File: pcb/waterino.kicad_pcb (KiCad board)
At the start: 2 copper layers, 49 x 84 mm, 50 parts, among them IC1 ATMEGA168A-P, P6 CONN_01X04, U1 LM7805CT, U2 MIC94090, U3 MAX6817, Y1 Crystal

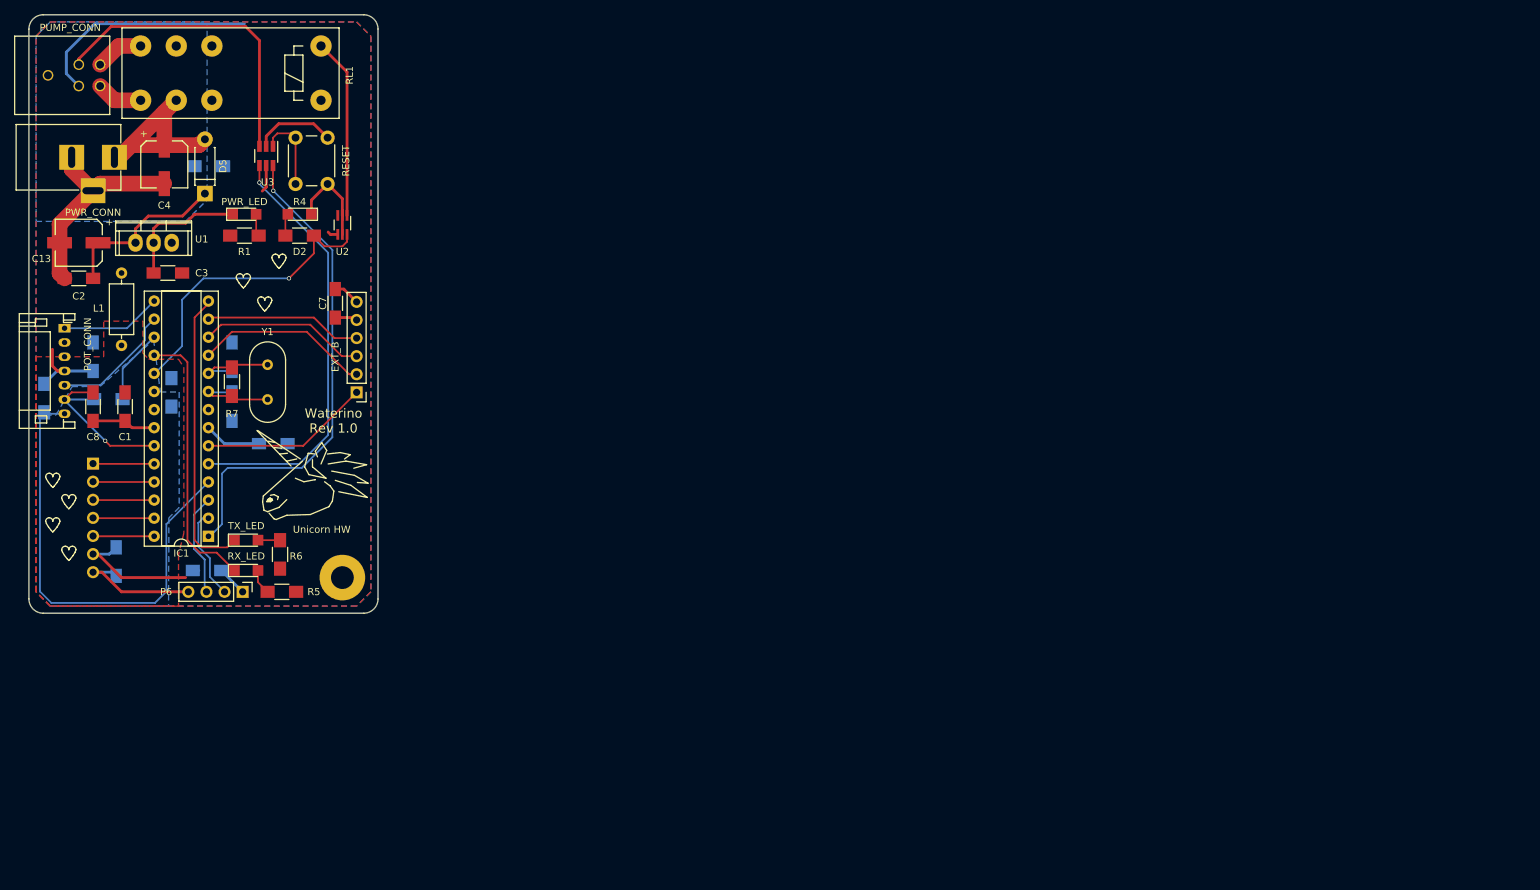
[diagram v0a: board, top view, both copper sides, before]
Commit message: wip
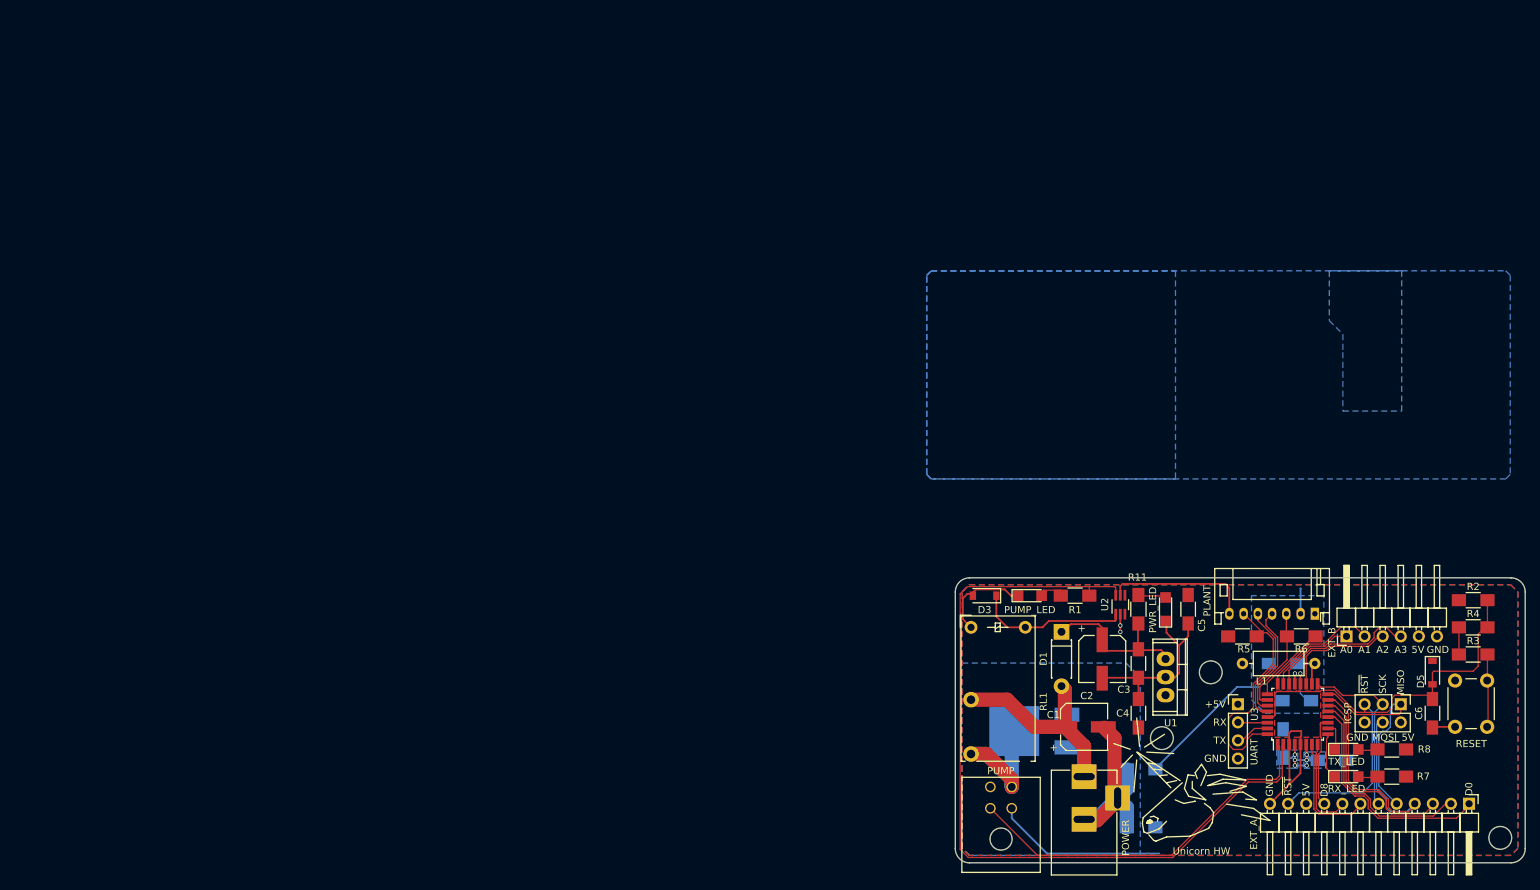
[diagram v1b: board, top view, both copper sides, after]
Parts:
- removed C10: 100nF, Capacitors_SMD:C_1206_HandSoldering
- removed C13: 100µF, Capacitors_SMD:CP_Elec_6.3x7.7
- removed C8: 22pF, Capacitors_SMD:C_1206_HandSoldering
- removed EXT_A: CONN_01X07, Pin_Headers:Pin_Header_Angled_1x07_Pitch2.54mm
- removed EXT_B: CONN_01X06, Pin_Headers:Pin_Header_Straight_1x06_Pitch2.54mm
- removed IC1: ATMEGA168A-P, Housings_DIP:DIP-28_W7.62mm_Socket
- removed P6: CONN_01X04, Pin_Headers:Pin_Header_Straight_1x04_Pitch2.54mm
- removed POT_CONN: CONN_01X07, Connectors_JST:JST_PH_S7B-PH-K_07x2.00mm_Angled
- removed PUMP_CONN: CONN_02X02, Connectors_Molex:Molex_Microfit3_Header_02x02_Angled_43045-040x
- removed PWR_CONN: BARREL_JACK, Connect:BARREL_JACK
- removed PWR_LED, RX_LED, TX_LED: LED, LEDs:LED_1206
- removed REF** (x7): HEARTS, HEARTS
- removed REF**: Unicorn HW, Unicorn HW
- removed REF**: MountingHole_3.2mm_M3_Pad, Mounting_Holes:MountingHole_3.2mm_M3_Pad
- removed RESET: SW_PUSH, Buttons_Switches_ThroughHole:SW_PUSH_6mm
- removed Y1: Crystal, Crystals:Crystal_HC49-U_Vertical
- added CON1: POWER, Connectors:BARREL_JACK, F.Cu at (182.1, 138.9)
- added D1: D, Diodes_THT:D_DO-41_SOD81_P7.62mm_Horizontal, F.Cu at (178.9, 118.6)
- added D3: D_Schottky, Diodes_SMD:D_SOD-123, F.Cu at (168.1, 113.5)
- added D4: PUMP_LED, LEDs:LED_1206, F.Cu at (174.5, 113.5)
- added D6: RX_LED, LEDs:LED_1206, F.Cu at (218.9, 138.9)
- added D7: TX_LED, LEDs:LED_1206, F.Cu at (218.9, 135.1)
- added D8: PWR_LED, LEDs:LED_1206, F.Cu at (193.5, 115.4)
- added J1: ICSP, Pin_Headers:Pin_Header_Straight_2x03_Pitch2.54mm, F.Cu at (226.6, 128.8)
- added J2: EXT_B, Pin_Headers:Pin_Header_Angled_1x06_Pitch2.54mm, F.Cu at (218.9, 119.3)
- added J3: EXT_A, Pin_Headers:Pin_Header_Angled_1x12_Pitch2.54mm, F.Cu at (236.1, 142.7)
- added LOGO: Unicorn HW, Logos:Unicorn HW, F.Cu at (189.1, 130.9)
- added MH1: MountingHole_3.2mm_M3, Mounting_Holes:MountingHole_3.2mm_M3, F.Cu at (193.0, 133.5)
- added MH2: MountingHole_3.2mm_M3, Mounting_Holes:MountingHole_3.2mm_M3, F.Cu at (199.9, 124.3)
- added MH3: MountingHole_3.2mm_M3, Mounting_Holes:MountingHole_3.2mm_M3, F.Cu at (240.5, 147.5)
- added P1: PUMP, Connectors_Molex:Molex_Microfit3_Header_02x02_Angled_43045-040x, F.Cu at (172.0, 143.4)
- added P2: PLANT, Connectors_JST:JST_PH_S7B-PH-K_07x2.00mm_Angled, F.Cu at (214.5, 116.1)
- added P3: UART, Pin_Headers:Pin_Header_Straight_1x04_Pitch2.54mm, F.Cu at (203.7, 128.8)
- added R11: 1.5K, Resistors_SMD:R_1206_HandSoldering, F.Cu at (189.7, 115.4)
- added R8: 150R, Resistors_SMD:R_1206_HandSoldering, F.Cu at (225.3, 135.1)
- added SW1: RESET, Buttons_Switches_THT:SW_PUSH_6mm, F.Cu at (234.2, 132.0)
- C1: value 100nF -> 100µF; footprint Capacitors_SMD:C_1206_HandSoldering -> Capacitors_SMD:CP_Elec_6.3x7.7
- C12: value 100nF -> 10nF
- C2: value 330nF -> 100µF; footprint Capacitors_SMD:C_1206_HandSoldering -> Capacitors_SMD:CP_Elec_6.3x7.7
- C3: value 10µF -> 100nF
- C4: value 100µF -> 100nF; footprint Capacitors_SMD:CP_Elec_6.3x7.7 -> Capacitors_SMD:C_1206_HandSoldering
- C5, C6: value 22pF -> 100nF; moved to F.Cu
- C7: moved to B.Cu
- D2: value LED -> D_Schottky_AKA; footprint LEDs:LED_1206 -> TO_SOT_Packages_SMD:TO-252-2_Rectifier; moved to B.Cu
- D5: value D -> D_Schottky; footprint Diodes_ThroughHole:D_DO-41_SOD81_P7.62mm_Horizontal -> Diodes_SMD:D_SOD-123
- R1: value 280 -> 1.5k
- R2: value 10k -> 4k7; moved to F.Cu
- R3: value 100k -> 150; moved to F.Cu
- R4: value 1.5k -> 150
- R5: value 145 -> 100k
- R6: value 145 -> 10k
- R7: value 1M -> 150R
- RL1: value FINDER-40.52 -> FINDER-32.21-x300; footprint Relays_ThroughHole:Relay_DPDT_Finder_40.52 -> Relays_THT:Relay_SPST_Finder_32.21-x300
- U3: value MAX6817 -> ATMEGA168-20AU; footprint TO_SOT_Packages_SMD:SOT-23-6_Handsoldering -> Housings_QFP:TQFP-32_7x7mm_Pitch0.8mm
- moved R3 203.8 mm to (236.7, 121.8), turned to 180 degrees
- moved R2 193.6 mm to (236.7, 114.2), turned to 180 degrees
- moved D5 185.0 mm to (231.0, 124.3), turned to 270 degrees
- moved C6 175.8 mm to (231.0, 130.0)
- moved R4 173.7 mm to (236.7, 118.0)
- moved R7 172.0 mm to (225.3, 138.9), turned to 180 degrees
- moved L1 166.6 mm to (204.3, 123.1), turned to 0 degrees
- moved C9 165.8 mm to (210.1, 134.3), turned to 90 degrees
- moved U3 164.6 mm to (212.1, 130.2), turned to 90 degrees
- moved C4 156.9 mm to (189.7, 130.0), turned to 90 degrees
- moved R10 155.9 mm to (190.1, 137.9), turned to 180 degrees
- moved U1 154.6 mm to (193.5, 125.0), turned to 270 degrees
- moved C7 153.9 mm to (216.9, 136.7), turned to 0 degrees
- moved C2 153.3 mm to (184.7, 122.4), turned to 270 degrees
- moved C11 151.6 mm to (210.1, 123.1)
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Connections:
- C1 pad 1: AVcc -> +12V
- C1 pad 2: AVss -> PGND
- C11 pad 1: Vcc -> AVcc
- C11 pad 2: GND -> AVss
- C12 pad 1: Vcc -> Net-(C12-Pad1)
- C12 pad 2: GND -> AVss
- C2 pad 1: /REG_PWR -> REG_PWR
- C2 pad 2: PGND -> GND
- C3 pad 1: Vcc -> REG_PWR
- C4 pad 1: +12V -> Vcc
- C4 pad 2: PGND -> GND
- C5 pad 1: GND -> Vcc
- C5 pad 2: /XTAL1 -> GND
- C6 pad 1: GND -> ~RESET
- C6 pad 2: /XTAL2 -> GND
- D2 pad 1: GND -> PGND
- D2 pad 2: Net-(D2-Pad2) -> /PUMP+
- D5 pad 1: /REG_PWR -> Vcc
- D5 pad 2: +12V -> ~RESET
- R1 pad 1: Vcc -> Net-(D4-Pad2)
- R1 pad 2: Net-(D1-Pad2) -> PUMP
- R10 pad 1: PGND -> AVss
- R10 pad 2: GND -> PGND
- R2 pad 1: MOISTURE -> ~RESET
- R2 pad 2: /MOIST+ -> Vcc
- R3 pad 1: Vcc -> Net-(R3-Pad1)
- R3 pad 2: ~OVRFLW -> Net-(R3-Pad2)
- R4 pad 1: Net-(D2-Pad2) -> Net-(R3-Pad2)
- R4 pad 2: PUMP -> ~RESET
- R5 pad 2: Net-(D3-Pad2) -> ~OVRFLW
- R6 pad 1: Vcc -> MOISTURE
- R6 pad 2: Net-(D4-Pad2) -> MOIST+
- R7 pad 1: /XTAL1 -> Vcc
- R7 pad 2: /XTAL2 -> Net-(D6-Pad2)
- R9 pad 1: AVss -> PGND
- U1 pad 1: /REG_PWR -> REG_PWR
- U3 pad 1: Net-(SW1-Pad1) -> ~LEVEL_ALERT
- U3 pad 2: GND -> PUMP
- U3 pad 3: /LVL_SWTCH -> GND
- U3 pad 4: LEVEL_ALERT -> Vcc
- U3 pad 5: Vcc -> GND
- U3 pad 6: RESET -> Vcc
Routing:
- net ~RESET: track 0.00 -> 76.4 mm
- net PUMP: track 42.3 -> 116.1 mm, vias 1 -> 0
- net RESET: track 68.9 -> 0.00 mm, vias 1 -> 0
- net LEVEL_ALERT: track 60.3 -> 0.00 mm, vias 1 -> 0
- net ~LEVEL_ALERT: track 0.00 -> 52.8 mm
- net MOSI: track 0.00 -> 44.9 mm
- net /LVL_SWTCH: track 43.7 -> 0.00 mm
- net TX_LED: track 40.8 -> 4.09 mm
- net Vcc: track 50.8 -> 17.9 mm, vias 0 -> 6
- net RX_LED: track 39.0 -> 6.69 mm
- net EXT_D0: track 0.00 -> 32.1 mm
- net ~OVRFLW: track 64.0 -> 33.0 mm
- net MISO: track 0.00 -> 30.1 mm
- net EXT_D1: track 0.00 -> 29.5 mm
- net EXT_D2: track 0.00 -> 27.7 mm
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- added copper zone on F.Cu, net GND
- added copper zone on B.Cu, net Vcc
- removed copper zone on F.Cu, net AVcc
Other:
- board size 49 x 84 mm -> 80 x 40 mm
- net class 12V: clearance 0.7 -> 0.2; trace_width 2.2 -> 2; via_dia 6 -> 0.6; via_drill 5 -> 0.4
- net class 5V added: clearance 0.1524, trace_width 0.254, via_dia 0.6, via_drill 0.4
- net class Default: clearance 0.2 -> 0.1524; trace_width 0.25 -> 0.1524
- net class Power removed
- rule pad_to_mask_clearance: 0.2 -> 0.35
- rule trace_clearance: 0.2 -> 0.1524
- rule trace_min: 0.2 -> 0.1524
- rule via_min_size: 0.4 -> 0.4524
- board text added: "+5V"
- board text added: "5V"
- board text added: "A0"
- board text added: "A1"
- board text added: "A2"
- board text added: "A3"
- board text added: "D0"
- board text added: "D8"
- board text added: "GND"
- board text added: "MISO"
- board text added: "MOSI"
- board text added: "Net classes: 5V Signal (Default) : 0.1524mm/0.1524mm (6/6mil). 1A max 100V max 5V Power: 0.254mm/0.1524mm (15.8/6mil). 1.4A max 100V max 12V Power: 2mm trace width 6.4A 0.2mm spacing (good for 100V)"
- board text added: "RX"
- board text added: "SCK"
- board text added: "Seed Studio: 2 layer, 1oz (35µm) Min track spacing/width 6mil (0.1524mm) Min pour spacing: 8 mil (0.2032mm) Min via-to-via: 12mil (0.3048mm) Min via ring: 6mil (0.1524mm) Min solder mask width: 0.35mm Min distance between copper and hole: 0.2mm/7.87mil Min pad to silk screen: 6mil (0.1524mm)"
- board text added: "TX"
- board text added: "~RST"
- board text removed: "Analog Block"
- board text removed: "Pump / 12V / Power Block"
- board text removed: "Waterino Rev 1.0"

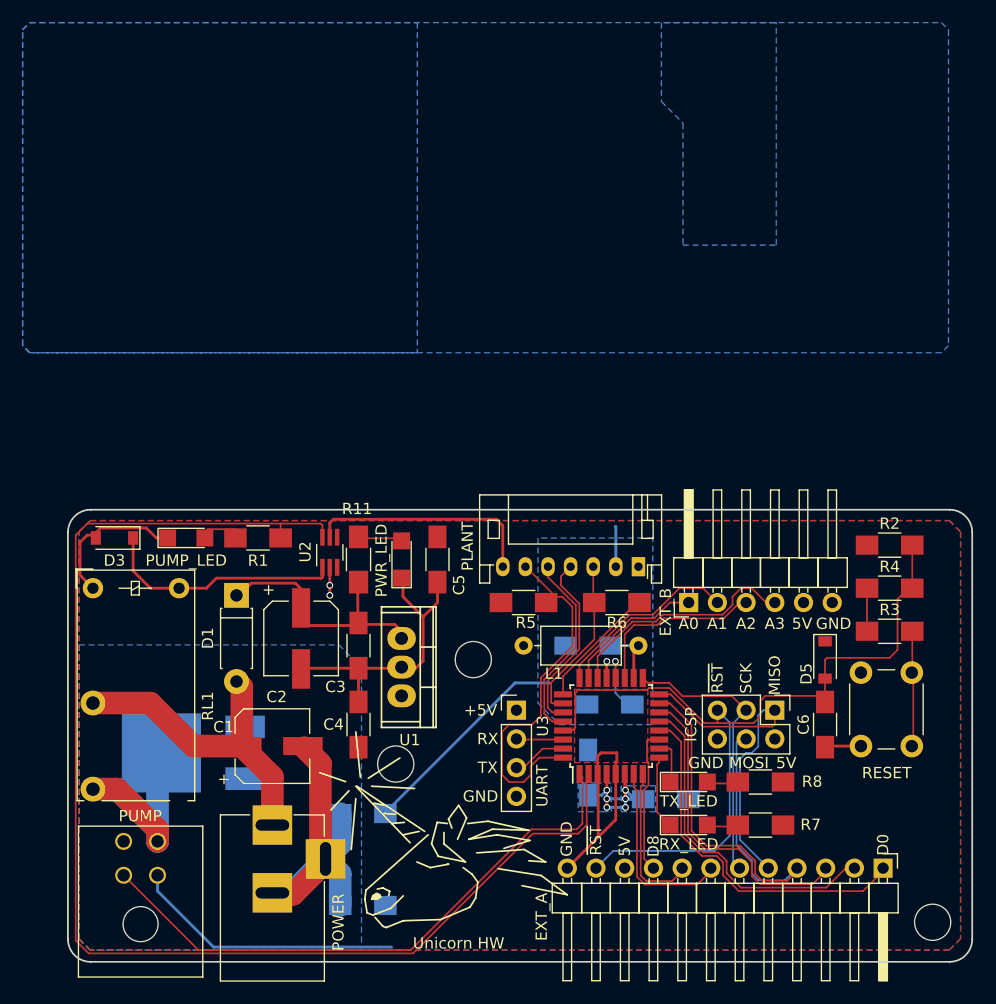
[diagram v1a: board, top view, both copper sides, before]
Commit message: Finally got it all together and ordered
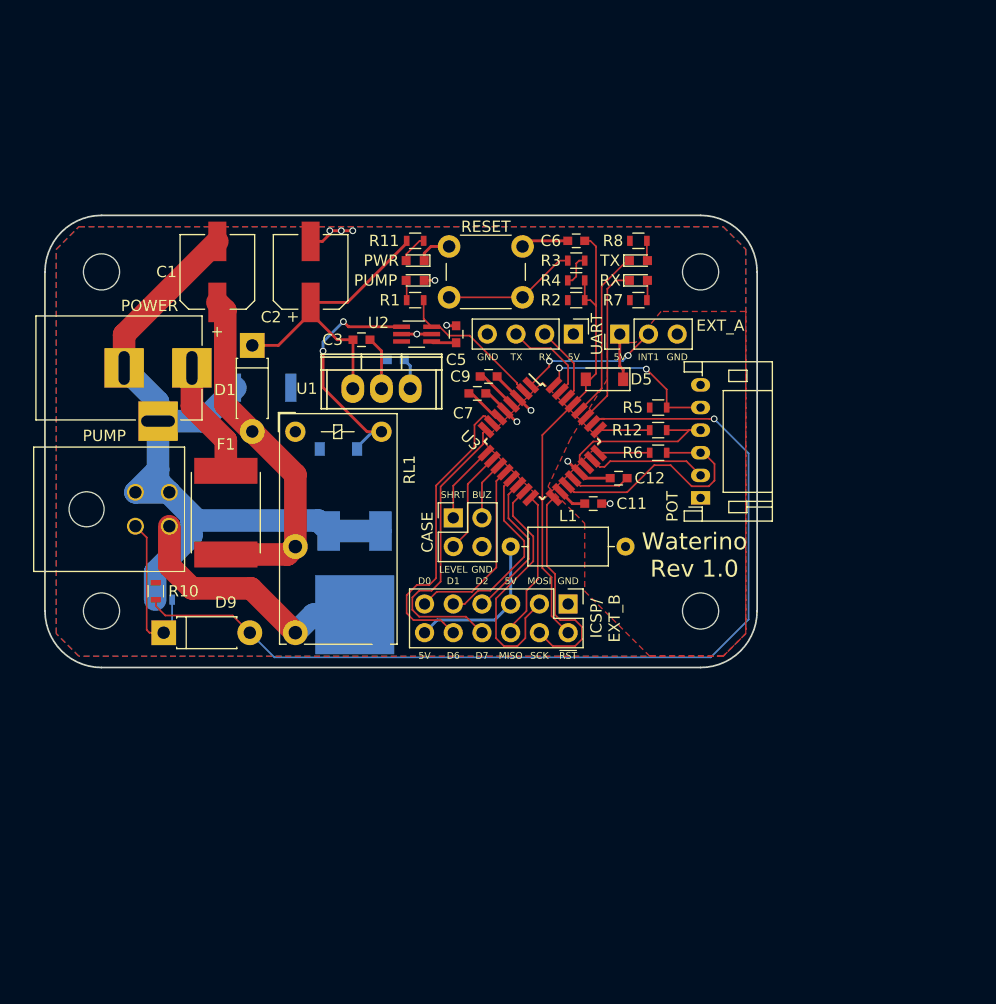
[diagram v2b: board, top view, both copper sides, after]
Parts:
- removed J1: ICSP, Pin_Headers:Pin_Header_Straight_2x03_Pitch2.54mm
- removed J2: EXT_B, Pin_Headers:Pin_Header_Angled_1x06_Pitch2.54mm
- removed J3: EXT_A, Pin_Headers:Pin_Header_Angled_1x12_Pitch2.54mm
- removed LOGO: Unicorn HW, Logos:Unicorn HW
- removed MH1, MH2, MH3: MountingHole_3.2mm_M3, Mounting_Holes:MountingHole_3.2mm_M3
- added D9: D, Diodes_ThroughHole:D_DO-41_SOD81_P7.62mm_Horizontal, F.Cu at (172.5, 121.9)
- added F1: FUSE, Fuse_Holders_and_Fuses:Fuse_SMD2920, F.Cu at (178.0, 111.3)
- added MH_LL: MountingHole_3.2mm_M3, Mounting_Holes:MountingHole_3.2mm_M3, F.Cu at (167.0, 120.0)
- added MH_LR: MountingHole_3.2mm_M3, Mounting_Holes:MountingHole_3.2mm_M3, F.Cu at (220.0, 120.0)
- added MH_UL: MountingHole_3.2mm_M3, Mounting_Holes:MountingHole_3.2mm_M3, F.Cu at (167.0, 90.0)
- added MH_UR: MountingHole_3.2mm_M3, Mounting_Holes:MountingHole_3.2mm_M3, F.Cu at (220.0, 90.0)
- added P4: CONN_02X06, Pin_Headers:Pin_Header_Straight_2x06_Pitch2.54mm, F.Cu at (208.3, 119.4)
- added P5: CONN_01X04, Pin_Headers:Pin_Header_Straight_2x02_Pitch2.54mm, F.Cu at (198.1, 111.8)
- added P6: CONN_01X03, Pin_Headers:Pin_Header_Straight_1x03_Pitch2.54mm, F.Cu at (212.9, 95.5)
- added R12: 5K11, Resistors_SMD:R_0603, F.Cu at (216.2, 104.0)
- added R13: 10K, Resistors_SMD:R_0603, B.Cu at (172.5, 119.0)
- C11, C12, C7, C9: footprint Capacitors_SMD:C_1206_HandSoldering -> Capacitors_SMD:C_0603; moved to F.Cu
- C3, C5, C6: footprint Capacitors_SMD:C_1206_HandSoldering -> Capacitors_SMD:C_0603
- C4: footprint Capacitors_SMD:C_1206_HandSoldering -> Capacitors_SMD:C_0603; moved to B.Cu
- D3: moved to B.Cu
- D4, D6, D7, D8: footprint LEDs:LED_1206 -> LEDs:LED_0603
- P2: footprint Connectors_JST:JST_PH_S7B-PH-K_07x2.00mm_Angled -> Connectors_JST:JST_PH_S6B-PH-K_06x2.00mm_Angled
- R1: value 1.5k -> 1.5K; footprint Resistors_SMD:R_1206_HandSoldering -> Resistors_SMD:R_0603
- R10: value 0 -> 10K; footprint Resistors_SMD:R_1206_HandSoldering -> Resistors_SMD:R_0603; moved to F.Cu
- R11, R3, R4: footprint Resistors_SMD:R_1206_HandSoldering -> Resistors_SMD:R_0603
- R2: value 4k7 -> 4K7; footprint Resistors_SMD:R_1206_HandSoldering -> Resistors_SMD:R_0603
- R5: value 100k -> 100K; footprint Resistors_SMD:R_1206_HandSoldering -> Resistors_SMD:R_0603
- R6: value 10k -> 10K; footprint Resistors_SMD:R_1206_HandSoldering -> Resistors_SMD:R_0603
- R7, R8: value 150R -> 150; footprint Resistors_SMD:R_1206_HandSoldering -> Resistors_SMD:R_0603
- R9: footprint Resistors_SMD:R_1206_HandSoldering -> Resistors_SMD:R_2010
- moved SW1 57.3 mm to (197.8, 87.8), turned to 0 degrees
- moved R8 49.1 mm to (214.5, 87.2), turned to 0 degrees
- moved D6 48.4 mm to (214.5, 90.8)
- moved C6 48.1 mm to (209.0, 87.2), turned to 180 degrees
- moved R7 47.7 mm to (214.5, 92.5), turned to 0 degrees
- moved R9 46.6 mm to (181.3, 100.2), turned to 180 degrees
- moved D7 46.3 mm to (214.5, 89.0)
- moved R3 42.9 mm to (209.0, 89.0), turned to 0 degrees
- moved C1 42.2 mm to (177.2, 90.0), turned to 90 degrees
- moved CON1 41.1 mm to (175.0, 98.5), turned to 0 degrees
- moved C7 39.6 mm to (200.2, 100.8)
- moved R4 38.9 mm to (209.0, 90.8)
- moved C9 36.1 mm to (201.2, 99.2), turned to 0 degrees
- moved R2 35.2 mm to (209.0, 92.5)
- moved P3 33.7 mm to (208.8, 95.5), turned to 270 degrees
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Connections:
- net REG_PWR renamed /REG_PWR
- net RX renamed /RX
- net TX renamed /TX
- C1 pad 1: +12V -> /+12V
- C1 pad 2: PGND -> /PGND
- C11 pad 2: AVss -> GND
- C12 pad 2: AVss -> GND
- CON1 pad 1: +12V -> /PWR
- CON1 pad 2: PGND -> /PGND
- CON1 pad 3: PGND -> /PGND
- D1 pad 2: +12V -> /+12V
- D2 pad 1: PGND -> /PGND
- D2 pad 3: PGND -> /PGND
- D6 pad 1: RX_LED -> /RX_LED
- D7 pad 1: TX_LED -> /TX_LED
- P1 pad 1: GND -> Net-(D9-Pad1)
- P1 pad 2: ~LEVEL_ALERT -> /PGND
- P1 pad 4: PGND -> /PGND
- P2 pad 1: Vcc -> GND
- P2 pad 2: GND -> MOIST-
- P2 pad 4: MOIST- -> THERM
- P2 pad 5: THERM -> ~OVRFLW
- P2 pad 6: ~OVRFLW -> GND
- R1 pad 1: Net-(D4-Pad2) -> PUMP
- R1 pad 2: PUMP -> Net-(D4-Pad2)
- R10 pad 1: AVss -> Vcc
- R10 pad 2: PGND -> ~LEVEL_ALERT
- R5 pad 1: Vcc -> ~OVRFLW
- R5 pad 2: ~OVRFLW -> AVcc
- R6 pad 1: MOISTURE -> MOIST+
- R6 pad 2: MOIST+ -> MOISTURE
- R9 pad 1: PGND -> GND
- R9 pad 2: GND -> /PGND
- RL1 pad 11: +12V -> /+12V
- U3 pad 1: ~LEVEL_ALERT -> INT1
- U3 pad 10: TX_LED -> LEVEL_LED
- U3 pad 11: EXT_D8 -> BUZZER
- U3 pad 19: EXT_A2 -> MOISTURE
- U3 pad 21: AVss -> GND
- U3 pad 22: EXT_A3 -> THERM
- U3 pad 23: EXT_A0 -> MOIST-
- U3 pad 24: EXT_A1 -> MOIST+
- U3 pad 25: MOIST+ -> THERM+
- U3 pad 26: MOISTURE -> ~LEVEL_ALERT
- U3 pad 27: MOIST- -> /RX_LED
- U3 pad 28: THERM -> /TX_LED
- U3 pad 9: RX_LED -> SHORT_LED
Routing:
- net PUMP: track 116.1 -> 13.3 mm
- net GND: track 114.7 -> 34.1 mm, vias 2 -> 10
- net /PGND: track 0.00 -> 72.8 mm
- net ~RESET: track 76.4 -> 41.5 mm
- net ~LEVEL_ALERT: track 52.8 -> 86.2 mm, vias 0 -> 1
- net PGND: track 31.4 -> 0.00 mm
- net /+12V: track 0.00 -> 30.9 mm
- net +12V: track 28.7 -> 0.00 mm
- net MOSI: track 44.9 -> 22.3 mm
- net EXT_A3: track 21.0 -> 0.00 mm
- net AVss: track 20.8 -> 0.00 mm, vias 1 -> 0
- net MISO: track 30.1 -> 13.2 mm
- net EXT_A1: track 16.7 -> 0.00 mm
- net ~OVRFLW: track 33.0 -> 16.8 mm, vias 0 -> 2
- net EXT_A2: track 15.8 -> 0.00 mm
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- added copper zone on F.Cu, net AVcc
- removed copper zone on B.Cu, net AVss
- removed copper zone on B.Cu, net PGND
- removed copper zone on B.Cu, net Vcc
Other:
- board size 80 x 40 mm -> 63 x 40 mm
- net class 12V: via_dia 0.6 -> 1; via_drill 0.4 -> 0.7
- rule pad_to_mask_clearance: 0.35 -> 0.1
- rule solder_mask_min_width: 0.35 -> 0.4
- board text added: "BUZ"
- board text added: "CASE"
- board text added: "D1"
- board text added: "D2"
- board text added: "D6"
- board text added: "D7"
- board text added: "EXT_A"
- board text added: "ICSP/ EXT_B"
- board text added: "INT1"
- board text added: "LEVEL"
- board text added: "POT"
- board text added: "POWER"
- board text added: "PUMP"
- board text added: "PWR"
- board text added: "RESET"
- board text added: "SHRT"
- board text added: "UART"
- board text added: "Waterino Rev 1.0"
- board text removed: "+5V"
- board text removed: "A0"
- board text removed: "A1"
- board text removed: "A2"
- board text removed: "A3"
- board text removed: "D8"
